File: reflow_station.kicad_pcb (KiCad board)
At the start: 2 copper layers, 6.5 x 0.7 mm, 252 parts, among them IC1 AMC23C10DWVR, IC2 MP100LGN-Z, J1 1731734, J10 DG301-5.0-02P-12-00A_H_, J11 USB_A, J12 USB_C_Receptacle_USB2.0_16P, J13 Conn_ARM_JTAG_SWD_10, J2 1707027, J3 1707027, J4 F52Q-1A7H1-11015, J5 1707027, J6 1707027, J7 DG301-5.0-02P-12-00A_H_, J8 DG301-5.0-02P-12-00A_H_, J9 DG301-5.0-02P-12-00A_H_, M1 Fan_CPU_4pin, M2 Fan_CPU_4pin, M3 Fan_CPU_4pin, M4 Fan_CPU_4pin, Q1 BTA16-600B, Q2 BTA16-600B, Q3 BTA16-600B, Q4 BTA16-600B, Q5 KSC1815YTA, SW2 SW_DIP_x08, SW3 SW_SPST, SW4 SW_SPST, SW5 SW_SPST, SW6 SW_Push, SW7 SW_SPDT, SW8 SW_SPDT, U1 TPS82130, U10 TPS2051BDBVR, U11 RCLAMP0504F.TCT, U12 STM32F469VITx, U13 RCLAMP0504F.TCT, U14 RCLAMP0504F.TCT, U2 RAC20-12SK, U3 MOC3023M, U4 MOC3023M, U5 TPS82130, U6 MOC3023M, U7 MOC3023M, U8 ADS1118IDGS, U9 ADS1118IDGS, Y1 25MHz, Y2 32.768kHz

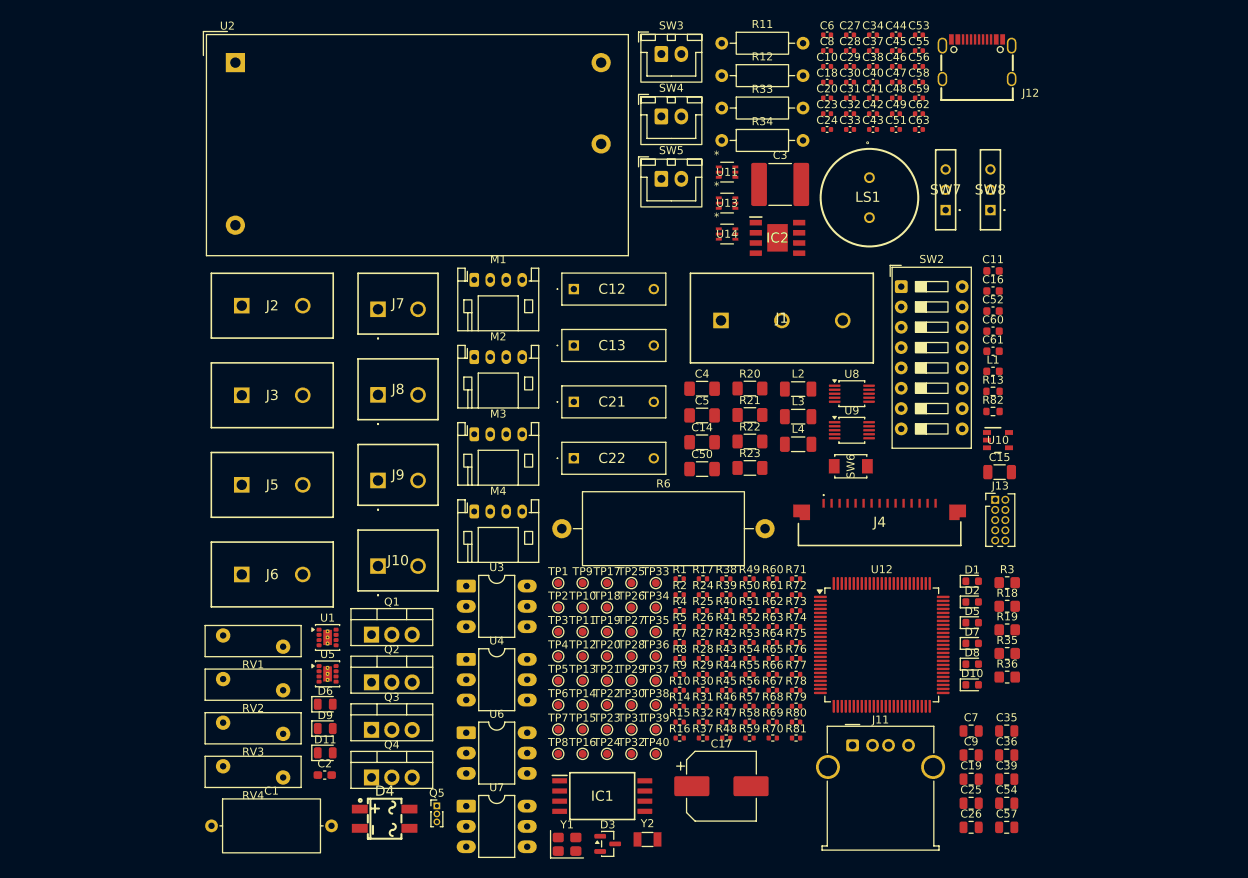
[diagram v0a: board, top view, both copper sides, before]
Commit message: feat: populate elements on board
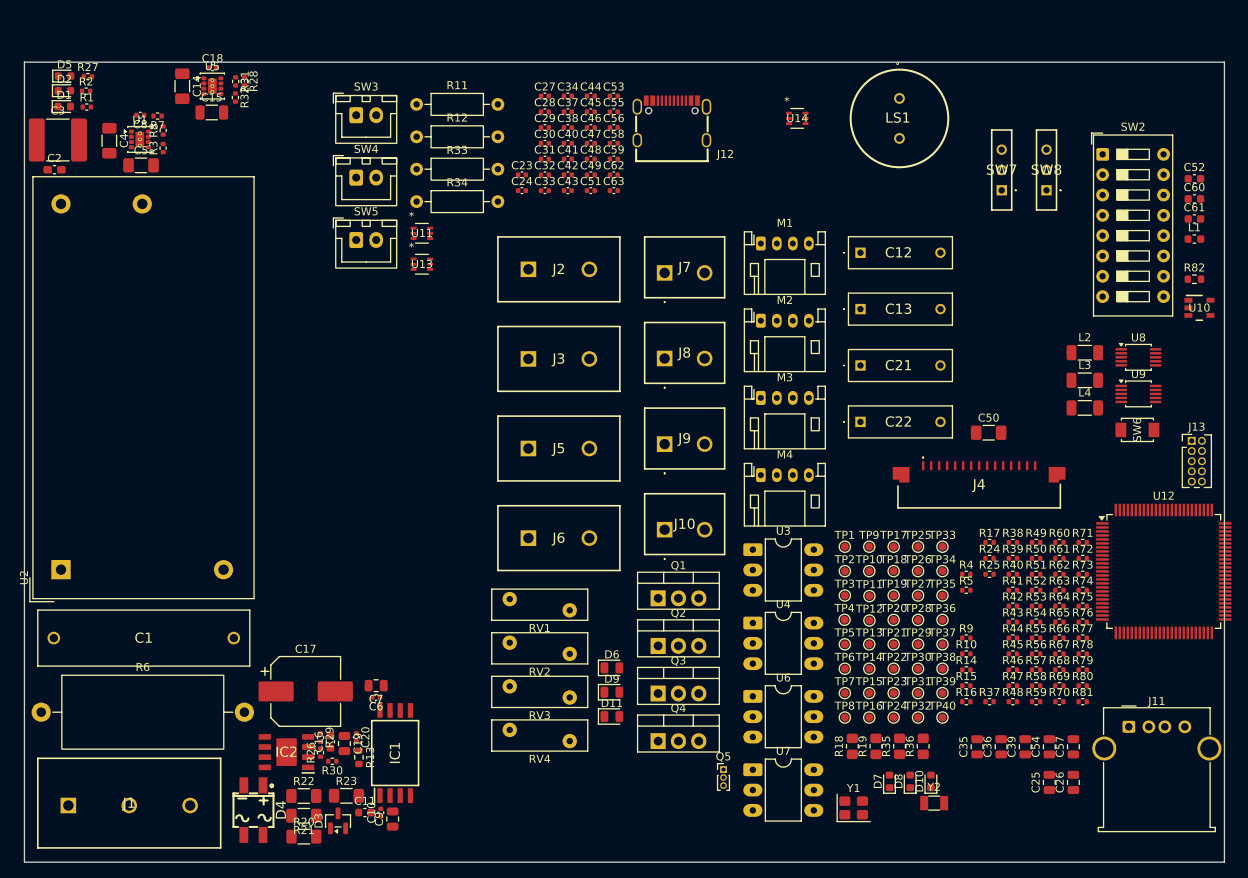
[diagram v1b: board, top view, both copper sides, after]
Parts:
- C1: footprint reflow_station_library:C_Axial_L12.0mm_D6.5mm_P15.00mm_Horizontal -> reflow_station_library:R474N31005001K
- R3: footprint reflow_station_library:R_0805_2012Metric_Pad1.20x1.40mm_HandSolder -> reflow_station_library:R_0402_1005Metric
- moved D5 132.4 mm to (78.6, 37.2)
- moved D2 130.2 mm to (78.6, 39.0)
- moved D1 128.1 mm to (78.6, 41.0)
- moved R3 118.7 mm to (90.9, 46.2), turned to 90 degrees
- moved C10 108.7 mm to (118.2, 129.3), turned to 90 degrees
- moved C15 108.3 mm to (97.0, 41.8)
- moved R27 104.5 mm to (81.5, 37.3)
- moved C11 103.7 mm to (116.2, 129.3)
- moved J1 101.6 mm to (79.1, 128.4)
- moved C16 100.2 mm to (111.8, 120.5), turned to 90 degrees
- moved C6 100.2 mm to (117.6, 114.9), turned to 180 degrees
- moved C20 99.2 mm to (115.1, 119.9), turned to -90 degrees
- moved R32 97.5 mm to (100.0, 39.9), turned to -90 degrees
- moved R31 97.5 mm to (100.0, 37.9), turned to -90 degrees
- moved R2 97.3 mm to (81.3, 39.1)
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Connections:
- D4 pad 2: /N -> GND1
- D4 pad 4: GND1 -> /N
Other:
- board size 6.5 x 0.7 mm -> 150 x 100 mm
- copper layers 2 -> 6
